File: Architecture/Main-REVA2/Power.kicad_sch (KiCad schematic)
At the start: 26 parts, among them J10 IN, J14 OUT_5V_ALI, J16 OUT_5V_PWR, J17 Barrel_Jack_Switch_Pin3Ring, Q2 PN2222A, Q3 IRF9540N, U3 MCP16311x-xMS

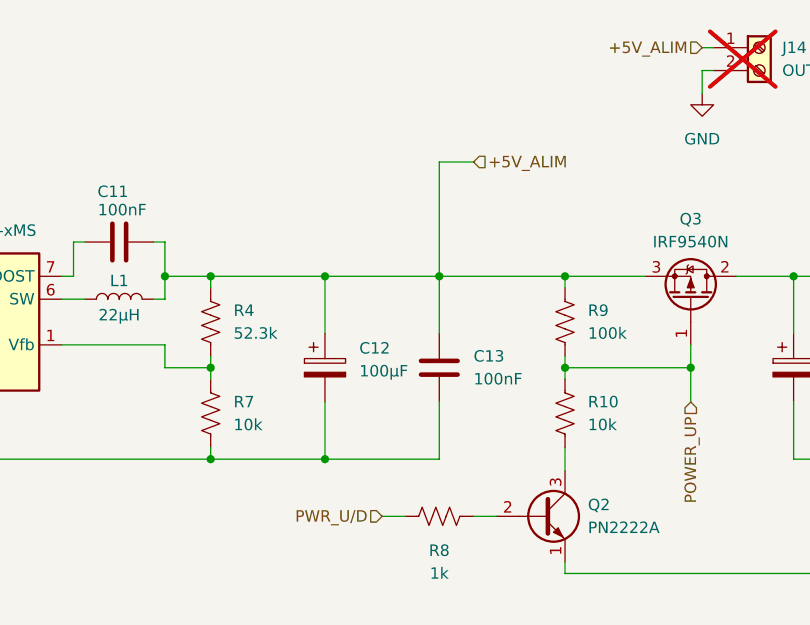
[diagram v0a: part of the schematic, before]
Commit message: update_01_02_2026
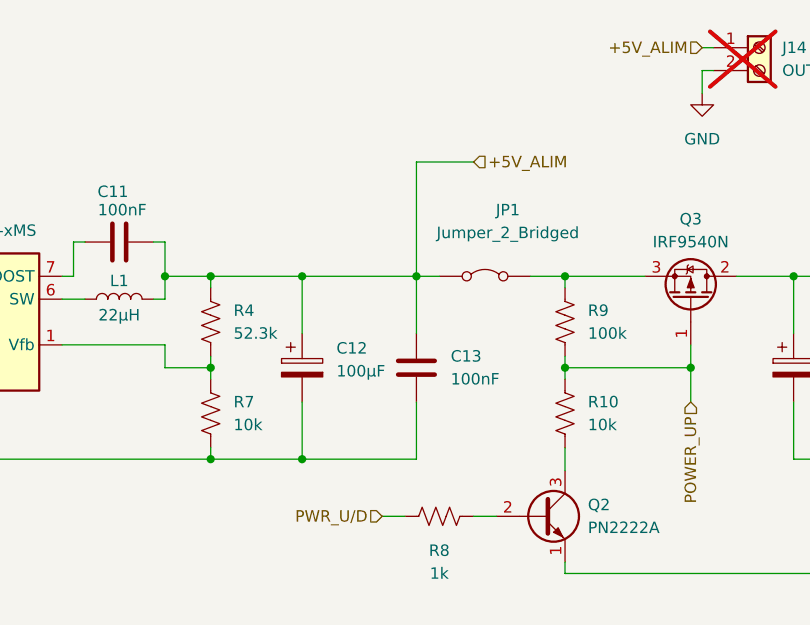
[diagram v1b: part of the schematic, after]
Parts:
- added JP1: Jumper_2_Bridged, Connector_PinHeader_2.54mm:PinHeader_1x02_P2.54mm_Vertical, symbol Jumper:Jumper_2_Bridged
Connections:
- net +5V_ALIM: now also JP1.1 (A); no longer Q3.3 (S), R9.1
- new net: JP1.2 (B), Q3.3 (S), R9.1
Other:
- moved on the sheet: C12, C13
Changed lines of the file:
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@@
 	)
 	(junction
-		(at 152.4 69.85)
+		(at 139.7 59.69)
 		(diameter 0)
 		(color 0 0 0 0)
 	)
 	(junction
-		(at 152.4 49.53)
+		(at 204.47 49.53)
 		(diameter 0)
 		(color 0 0 0 0)
 	)
 	(junction
-		(at 139.7 59.69)
+		(at 218.44 69.85)
 		(diameter 0)
 		(color 0 0 0 0)
 	)
 	(junction
-		(at 204.47 49.53)
+		(at 139.7 69.85)
 		(diameter 0)
 		(color 0 0 0 0)
 	)
 	(junction
-		(at 218.44 69.85)
+		(at 134.62 49.53)
 		(diameter 0)
 		(color 0 0 0 0)
 	)
 	(junction
-		(at 139.7 69.85)
+		(at 162.56 49.53)
 		(diameter 0)
 		(color 0 0 0 0)
 	)
 	(junction
-		(at 134.62 49.53)
+		(at 218.44 49.53)
 		(diameter 0)
 		(color 0 0 0 0)
 	)
 	(junction
-		(at 218.44 49.53)
+		(at 179.07 49.53)
 		(diameter 0)
 		(color 0 0 0 0)
@@
 	)
 	(junction
-		(at 71.12 124.46)
+		(at 149.86 49.53)
 		(diameter 0)
 		(color 0 0 0 0)
 	)
 	(junction
-		(at 82.55 69.85)
+		(at 71.12 124.46)
 		(diameter 0)
 		(color 0 0 0 0)
 	)
 	(junction
-		(at 165.1 49.53)
+		(at 82.55 69.85)
 		(diameter 0)
 		(color 0 0 0 0)
 	)
 	(junction
-		(at 66.04 69.85)
+		(at 149.86 69.85)
 		(diameter 0)
 		(color 0 0 0 0)
 	)
 	(junction
-		(at 69.85 49.53)
+		(at 66.04 69.85)
 		(diameter 0)
 		(color 0 0 0 0)
 	)
 	(junction
-		(at 179.07 49.53)
+		(at 69.85 49.53)
 		(diameter 0)
 		(color 0 0 0 0)
@@
 	(wire
 		(pts
-			(xy 95.25 52.07) (xy 102.87 52.07)
+			(xy 175.26 49.53) (xy 179.07 49.53)
 		)
 		(stroke
@@
 	(wire
 		(pts
-			(xy 179.07 49.53) (xy 165.1 49.53)
+			(xy 95.25 52.07) (xy 102.87 52.07)
 		)
 		(stroke
@@
 	(wire
 		(pts
-			(xy 165.1 69.85) (xy 152.4 69.85)
+			(xy 139.7 59.69) (xy 139.7 60.96)
 		)
 		(stroke
@@
 	(wire
 		(pts
-			(xy 139.7 59.69) (xy 139.7 60.96)
+			(xy 139.7 59.69) (xy 139.7 58.42)
 		)
 		(stroke
@@
 	(wire
 		(pts
-			(xy 139.7 59.69) (xy 139.7 58.42)
+			(xy 149.86 49.53) (xy 139.7 49.53)
+		)
+		(stroke
+			(width 0)
+			(type default)
+		)
+	)
+	(wire
+		(pts
+			(xy 149.86 69.85) (xy 162.56 69.85)
 		)
 		(stroke
@@
 	(wire
 		(pts
+			(xy 162.56 49.53) (xy 165.1 49.53)
+		)
+		(stroke
+			(width 0)
+			(type default)
+		)
+	)
+	(wire
+		(pts
 			(xy 134.62 49.53) (xy 134.62 52.07)
 		)
@@
 	(wire
 		(pts
-			(xy 139.7 69.85) (xy 152.4 69.85)
+			(xy 139.7 69.85) (xy 149.86 69.85)
 		)
 		(stroke
@@
 	(wire
 		(pts
-			(xy 165.1 36.83) (xy 165.1 49.53)
+			(xy 162.56 36.83) (xy 162.56 49.53)
 		)
 		(stroke
@@
 	(wire
 		(pts
-			(xy 165.1 36.83) (xy 168.91 36.83)
+			(xy 162.56 36.83) (xy 168.91 36.83)
 		)
 		(stroke
@@
 	(wire
 		(pts
-			(xy 165.1 49.53) (xy 165.1 55.88)
+			(xy 162.56 49.53) (xy 162.56 55.88)
 		)
 		(stroke
@@
 	(wire
 		(pts
-			(xy 152.4 49.53) (xy 139.7 49.53)
+			(xy 149.86 49.53) (xy 162.56 49.53)
 		)
 		(stroke
@@
 	(wire
 		(pts
-			(xy 165.1 49.53) (xy 152.4 49.53)
-		)
-		(stroke
-			(width 0)
-			(type default)
-		)
-	)
-	(wire
-		(pts
 			(xy 204.47 63.5) (xy 204.47 69.85)
 		)
@@
 	(wire
 		(pts
-			(xy 165.1 63.5) (xy 165.1 69.85)
+			(xy 162.56 63.5) (xy 162.56 69.85)
 		)
 		(stroke
@@
 	(wire
 		(pts
-			(xy 152.4 63.5) (xy 152.4 69.85)
+			(xy 149.86 63.5) (xy 149.86 69.85)
 		)
 		(stroke
@@
 	(wire
 		(pts
-			(xy 152.4 55.88) (xy 152.4 49.53)
+			(xy 149.86 55.88) (xy 149.86 49.53)
 		)
 		(stroke
@@
 	(symbol
 		(lib_id "Device:C_Polarized")
-		(at 152.4 59.69 0)
+		(at 149.86 59.69 0)
 		(unit 1)
 		(exclude_from_sim no)
@@
 		(fields_autoplaced yes)
 		(property "Reference" "C12"
-			(at 156.21 57.5309 0)
+			(at 153.67 57.5309 0)
 			(effects
 				(font
@@
 		)
 		(property "Value" "100µF"
-			(at 156.21 60.0709 0)
+			(at 153.67 60.0709 0)
 			(effects
 				(font
@@
 		)
 		(property "Footprint" "CollecteurDonne:C_Radial_D10.0mm_H16.0mm_P5.00mm"
-			(at 153.3652 63.5 0)
+			(at 150.8252 63.5 0)
 			(effects
 				(font
@@
 		)
 		(property "Datasheet" "~"
-			(at 152.4 59.69 0)
+			(at 149.86 59.69 0)
 			(effects
 				(font
@@
 		)
 		(property "Description" "Polarized capacitor"
-			(at 152.4 59.69 0)
+			(at 149.86 59.69 0)
 			(effects
 				(font
@@
 		)
 		(property "Fabricant" "Vishay"
-			(at 152.4 59.69 0)
+			(at 149.86 59.69 0)
 			(effects
 				(font
@@
 		)
 		(property "Fournisseur" "RS"
-			(at 152.4 59.69 0)
+			(at 149.86 59.69 0)
 			(effects
 				(font
@@
 		)
 		(property "Ref Fabricant" "MAL215373101E3"
-			(at 152.4 59.69 0)
+			(at 149.86 59.69 0)
 			(effects
 				(font
@@
 		)
 		(property "Ref Fournisseur" "280-6780P"
-			(at 152.4 59.69 0)
+			(at 149.86 59.69 0)
 			(effects
 				(font
@@
 		)
 		(property "Sim.Type" ""
-			(at 152.4 59.69 0)
+			(at 149.86 59.69 0)
 			(effects
 				(font
@@
 	)
 	(symbol
+		(lib_id "Jumper:Jumper_2_Bridged")
+		(at 170.18 49.53 0)
+		(unit 1)
+		(exclude_from_sim no)
+		(in_bom yes)
+		(on_board yes)
+		(dnp no)
+		(property "Reference" "JP1"
+			(at 172.72 42.164 0)
+			(effects
+				(font
+					(size 1.27 1.27)
+				)
+			)
+		)
+		(property "Value" "Jumper_2_Bridged"
+			(at 172.72 44.704 0)
+			(effects
+				(font
+					(size 1.27 1.27)
+				)
+			)
+		)
+		(property "Footprint" "Connector_PinHeader_2.54mm:PinHeader_1x02_P2.54mm_Vertical"
+			(at 170.18 49.53 0)
+			(effects
+				(font
+					(size 1.27 1.27)
+				)
+				(hide yes)
+			)
+		)
+		(property "Datasheet" "~"
+			(at 170.18 49.53 0)
+			(effects
+				(font
+					(size 1.27 1.27)
+				)
+				(hide yes)
+			)
+		)
+		(property "Description" "Jumper, 2-pole, closed/bridged"
+			(at 170.18 49.53 0)
+			(effects
+				(font
+					(size 1.27 1.27)
+				)
+				(hide yes)
+			)
+		)
+		(pin "1"
+		)
+		(pin "2"
+		)
+		(instances
+			(project ""
+				(path "/77f264da-4c84-4b0c-9d20-4392731765e6/8078826c-4446-4e50-a209-45fcf7cbe7e4"
+					(reference "JP1")
+					(unit 1)
+				)
+			)
+		)
+	)
+	(symbol
 		(lib_id "Connector:Screw_Terminal_01x02")
 		(at 252.73 25.4 0)
@@
 	(symbol
 		(lib_id "Device:C")
-		(at 165.1 59.69 0)
+		(at 162.56 59.69 0)
 		(unit 1)
 		(exclude_from_sim no)
@@
 		(dnp no)
 		(property "Reference" "C13"
-			(at 168.91 58.4199 0)
+			(at 166.37 58.4199 0)
 			(effects
 				(font
@@
 		)
 		(property "Value" "100nF"
-			(at 168.91 60.96 0)
+			(at 166.37 60.96 0)
 			(effects
 				(font
@@
 		)
 		(property "Footprint" "CollecteurDonne:C_Disc_D5.0mm_W2.5mm_P5.00mm"
-			(at 166.0652 63.5 0)
+			(at 163.5252 63.5 0)
 			(effects
 				(font
@@
 		)
 		(property "Datasheet" "~"
-			(at 165.1 59.69 0)
+			(at 162.56 59.69 0)
 			(effects
 				(font
@@
 		)
 		(property "Description" "Unpolarized capacitor"
-			(at 165.1 59.69 0)
+			(at 162.56 59.69 0)
 			(effects
 				(font
@@
 		)
 		(property "Fabricant" "KEMET"
-			(at 165.1 59.69 0)
+			(at 162.56 59.69 0)
 			(effects
 				(font
@@
 		)
 		(property "Fournisseur" "RS"
-			(at 165.1 59.69 0)
+			(at 162.56 59.69 0)
 			(effects
 				(font
@@
 		)
 		(property "Ref Fabricant" "C0805C104K4RACTU"
-			(at 165.1 59.69 0)
+			(at 162.56 59.69 0)
 			(effects
 				(font
@@
 		)
 		(property "Ref Fournisseur" "648-0957"
-			(at 165.1 59.69 0)
+			(at 162.56 59.69 0)
 			(effects
 				(font
@@
 		)
 		(property "Sim.Type" ""
-			(at 165.1 59.69 0)
+			(at 162.56 59.69 0)
 			(effects
 				(font
